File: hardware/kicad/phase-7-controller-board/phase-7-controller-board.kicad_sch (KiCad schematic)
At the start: 35 parts, among them J1 MONITOR_INPUT, J2 PI_GPIO_HEADER, J3 INTER_BOARD, U1 TLV9064IDR, U2 ADS1015IDGSR, U3 74LVC1G17GW, U4 74LVC1G17GW, U5 MC74HC4066ADTR2G, U6 74LVC1G66LT05ARCQ

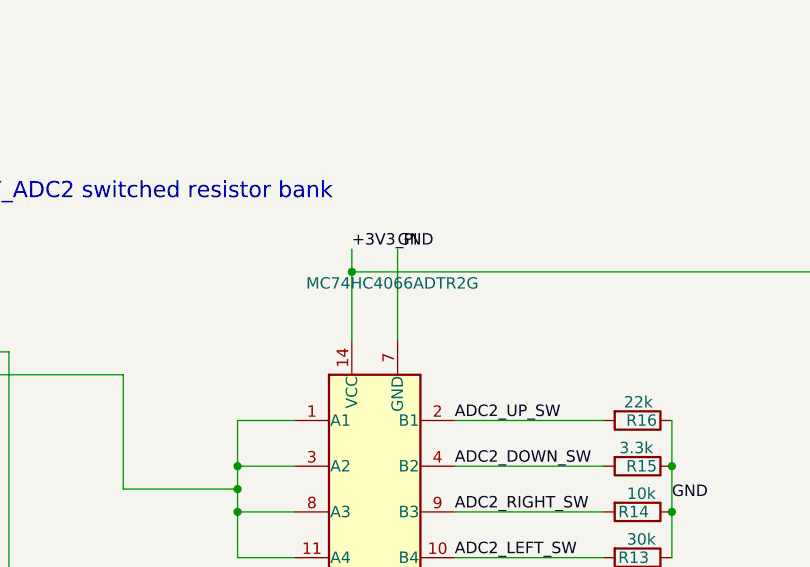
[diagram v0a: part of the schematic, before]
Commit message: Phase 7 WIP
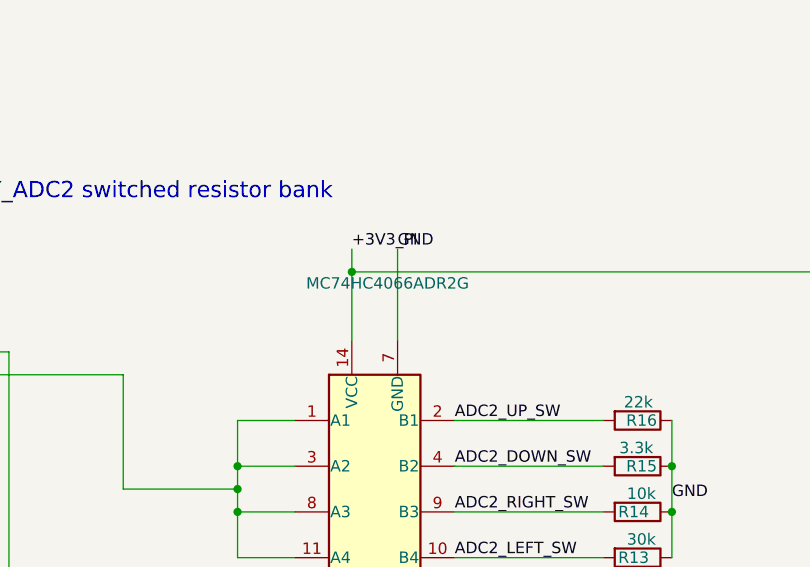
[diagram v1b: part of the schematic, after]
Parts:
- U5: value MC74HC4066ADTR2G -> MC74HC4066ADR2G; footprint Package_SO:TSSOP-14_4.4x5mm_P0.65mm -> Package_SO:SOIC-14_3.9x8.7mm_P1.27mm; LCSC (none) -> C233612; MPN MC74HC4066ADTR2G -> MC74HC4066ADR2G
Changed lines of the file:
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@@
 			)
 		)
-		(property "Value" "MC74HC4066ADTR2G"
+		(property "Value" "MC74HC4066ADR2G"
 			(at 354.1400 48.26 0)
 			(show_name no)
@@
 			)
 		)
-		(property "Footprint" "Package_SO:TSSOP-14_4.4x5mm_P0.65mm"
+		(property "Footprint" "Package_SO:SOIC-14_3.9x8.7mm_P1.27mm"
 			(at 361.7600 71.12 0)
 			(hide yes)
@@
 			)
 		)
-		(property "MPN" "MC74HC4066ADTR2G"
+		(property "MPN" "MC74HC4066ADR2G"
 			(at 368.0000 83.82 0)
 			(hide yes)
 			(show_name no)
+			(do_not_autoplace no)
+			(effects
+				(font
+					(size 1.27 1.27)
+				)
+				(justify left)
+			)
+		)
+		(property "LCSC" "C233612"
+			(at 368.0000 81.28 0)
+			(hide yes)
+			(show_name no)
